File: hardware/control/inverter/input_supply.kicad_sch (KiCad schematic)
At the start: 20 parts, among them J4 RJ45, J5 RJ45, J6 RJ45, U10 LM7815_TO220, U11 LM7815_TO220, U12 L7805, U14 74HC74, U20 74LS08, U8 74HC14

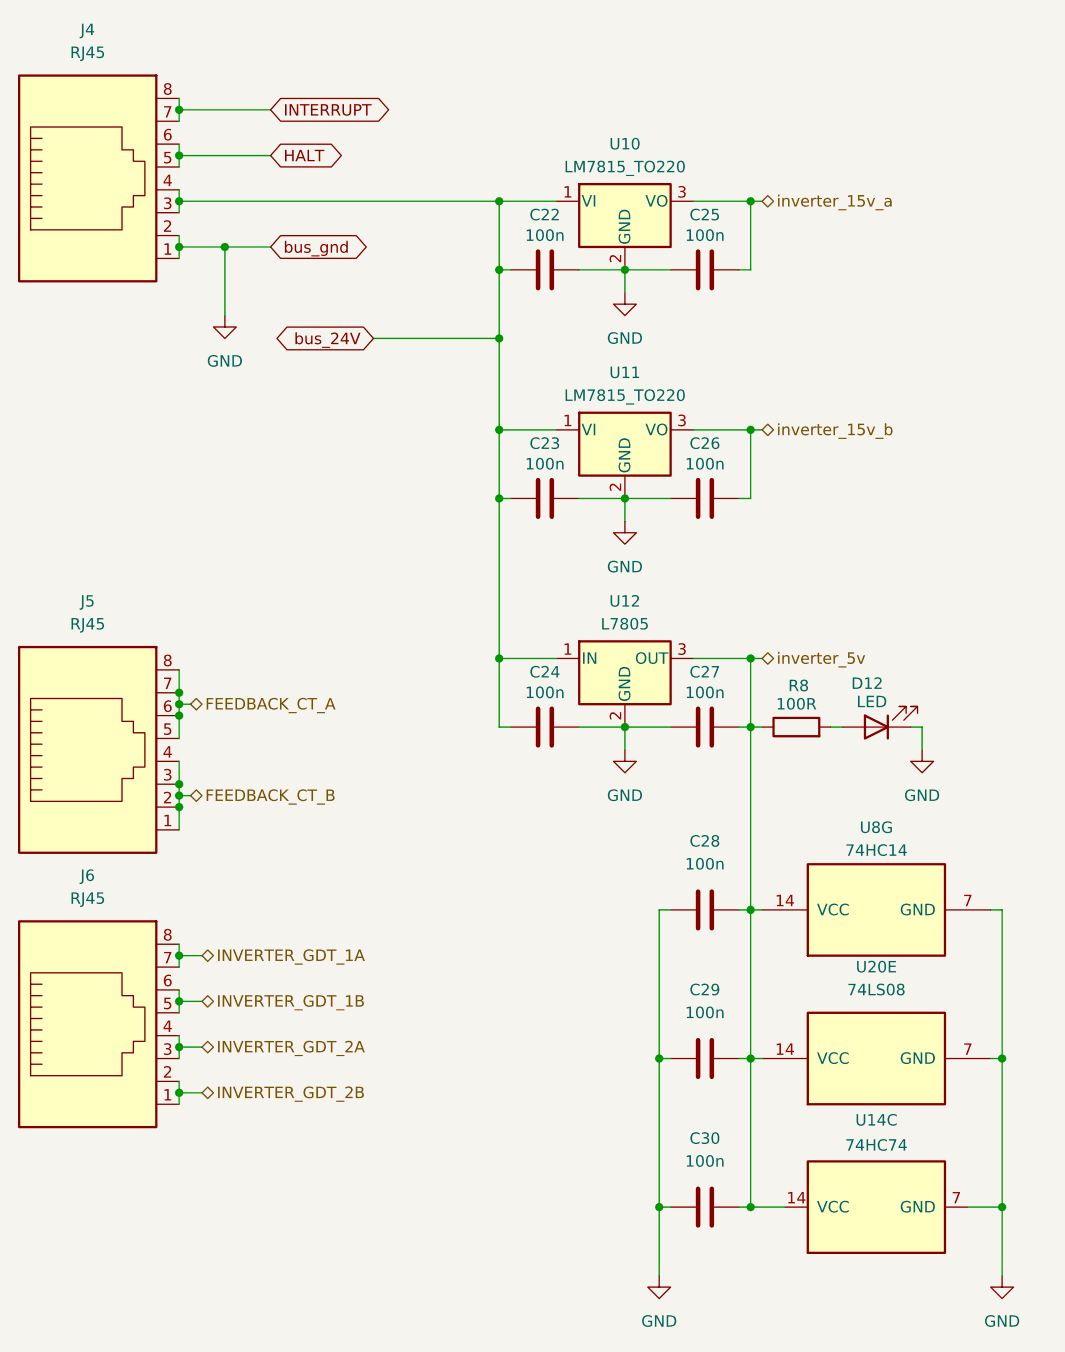
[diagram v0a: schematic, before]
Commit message: idk some changes
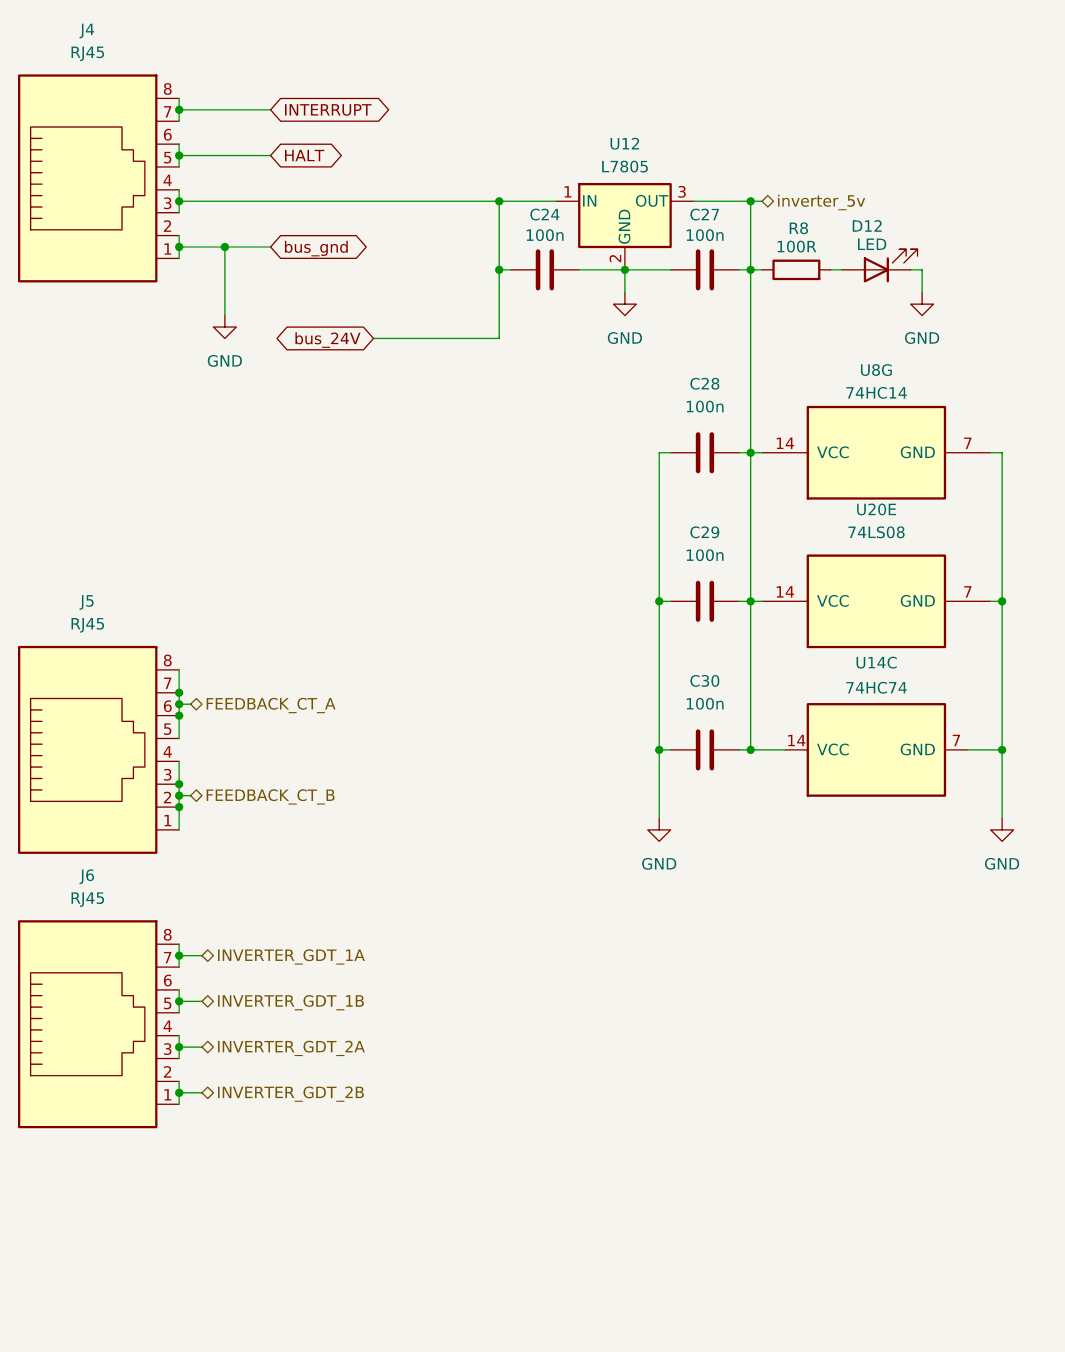
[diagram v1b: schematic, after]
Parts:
- removed C22, C23, C25, C26: 100n, symbol Device:C
- removed U10, U11: LM7815_TO220, Package_TO_SOT_THT:TO-220-3_Vertical, symbol Regulator_Linear:LM7815_TO220
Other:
- moved on the sheet: C24, C27, C28, C29, C30, D12, R8, U12, U14C, U20E, U8G

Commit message: completed-ish inverter board, probably not, but anyway
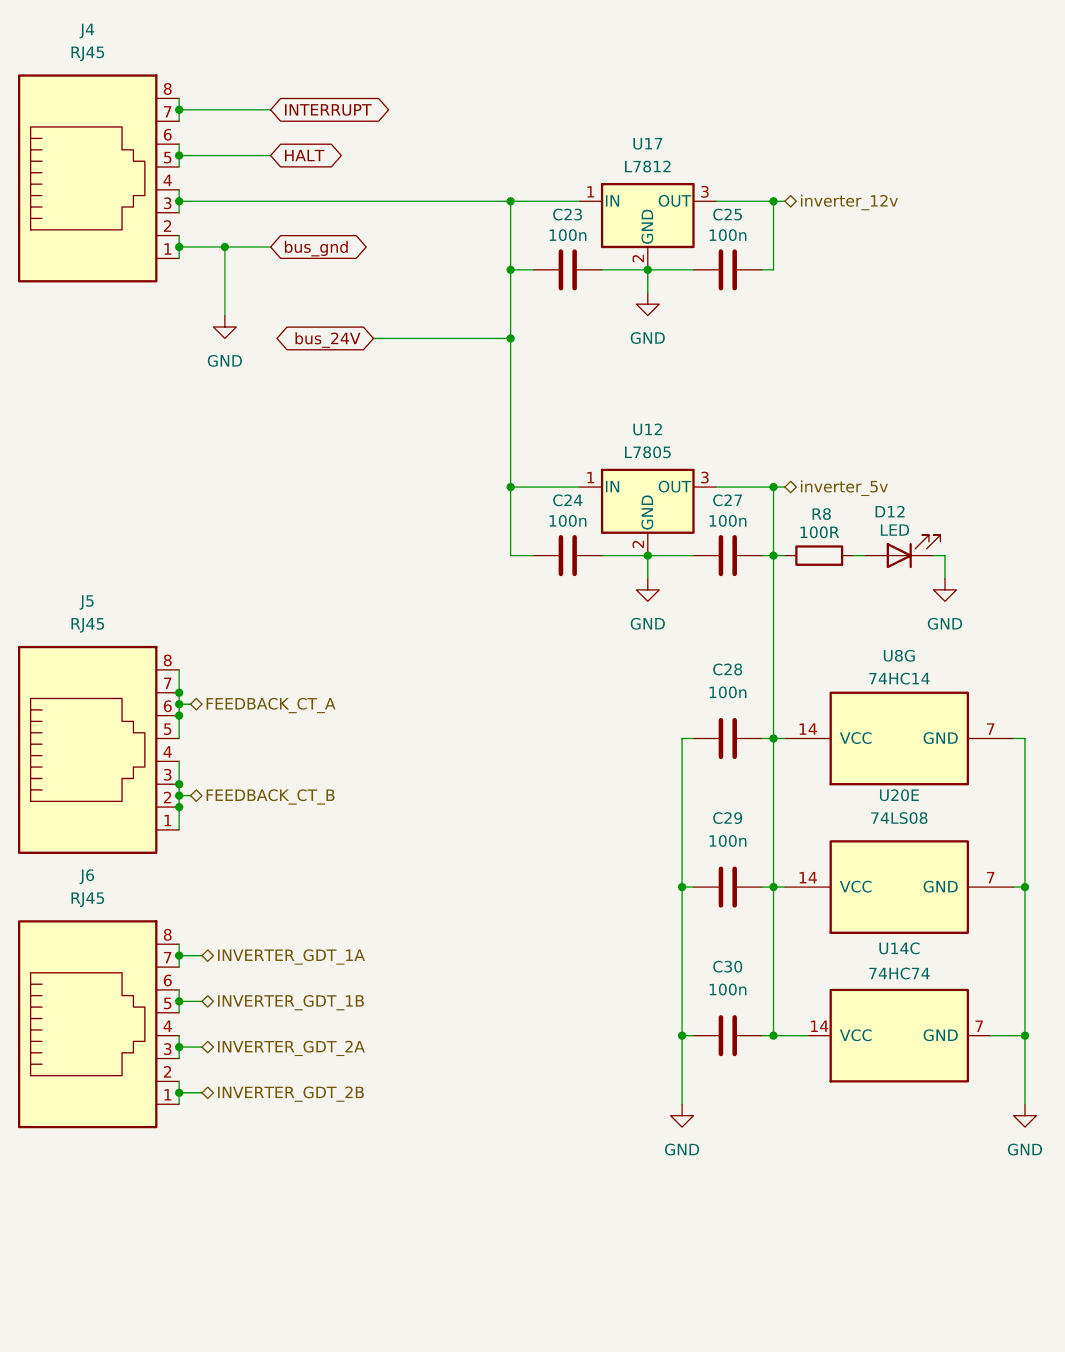
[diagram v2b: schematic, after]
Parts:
- added C23, C25: 100n, symbol Device:C
- added U17: L7812, symbol Regulator_Linear:L7812
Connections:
- net GND: now also C23.2, C25.1, U17.2 (GND)
- net bus_24V: now also C23.1, U17.1 (IN)
- new net inverter_12v: C25.2, U17.3 (OUT)
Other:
- moved on the sheet: C24, C27, C28, C29, C30, D12, R8, U12, U14C, U20E, U8G
